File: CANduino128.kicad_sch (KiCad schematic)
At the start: 37 parts, among them J1 Conn_02x32_Row_Letter_First, J2 Conn_01x10, U1 AVR-H128-CAN, U2 74AHC373

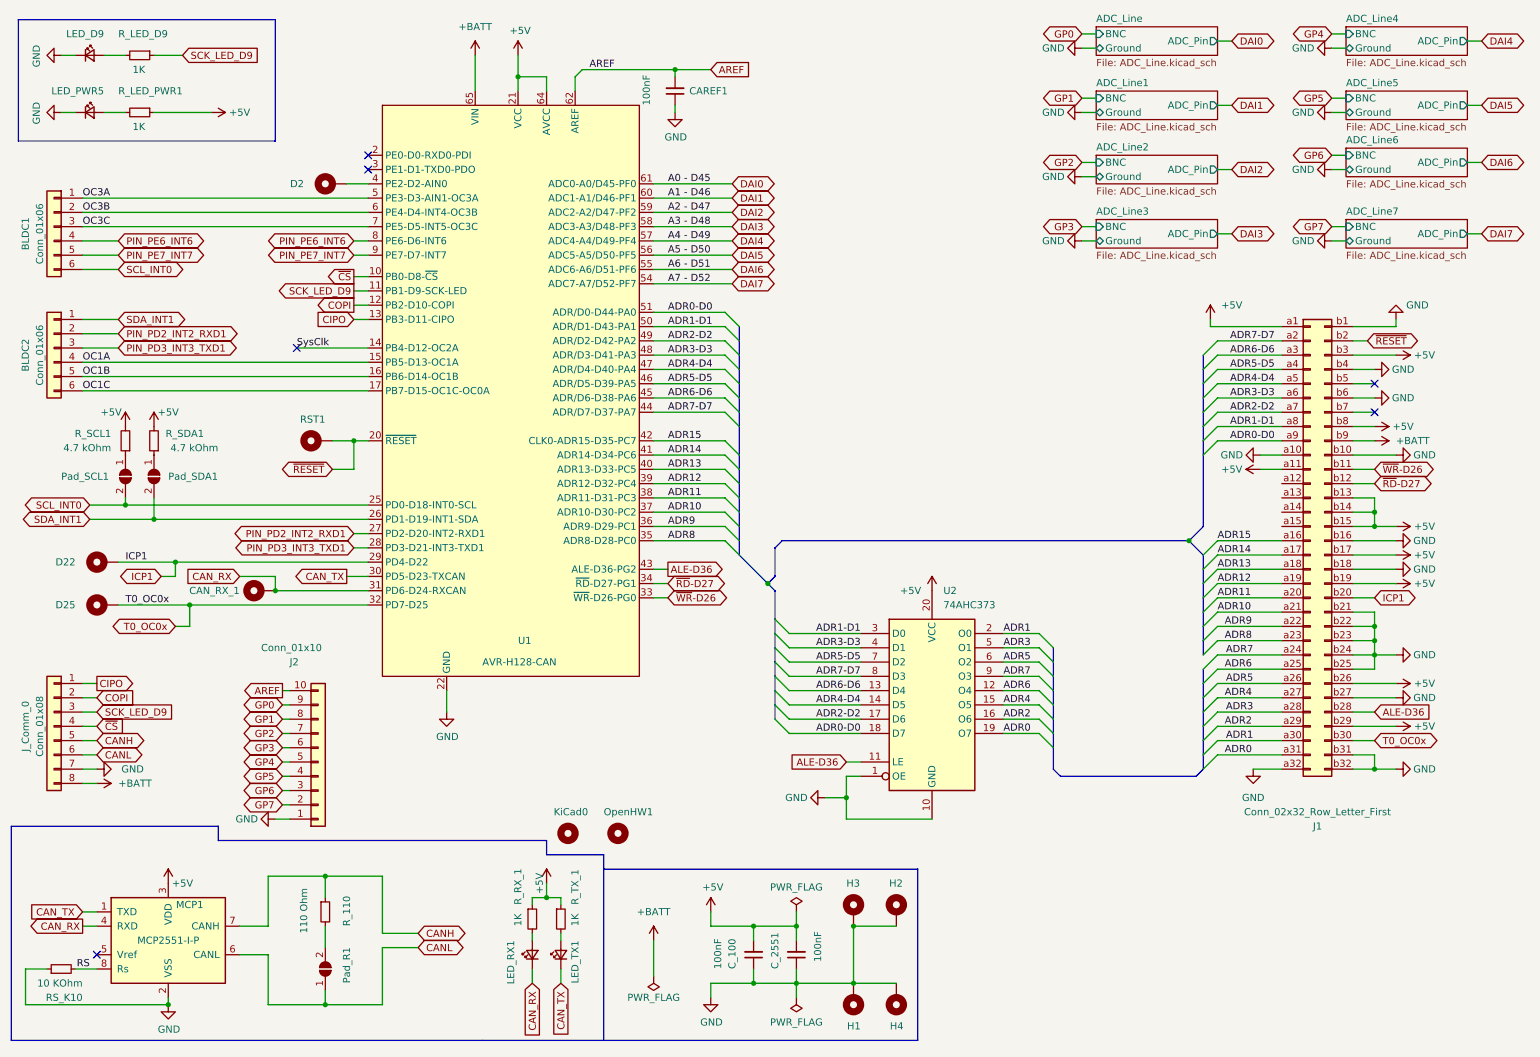
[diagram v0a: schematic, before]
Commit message: git-svn-id: file:///D%5C00%20-%20Dev%20&%20Calculs%5CRepoTortoiseSVN_PCB%5CCANduino128/branches/CANduino128%20-%20v3.x@78 67ddf66f-3787-a644-8df7-7746e21a92b3
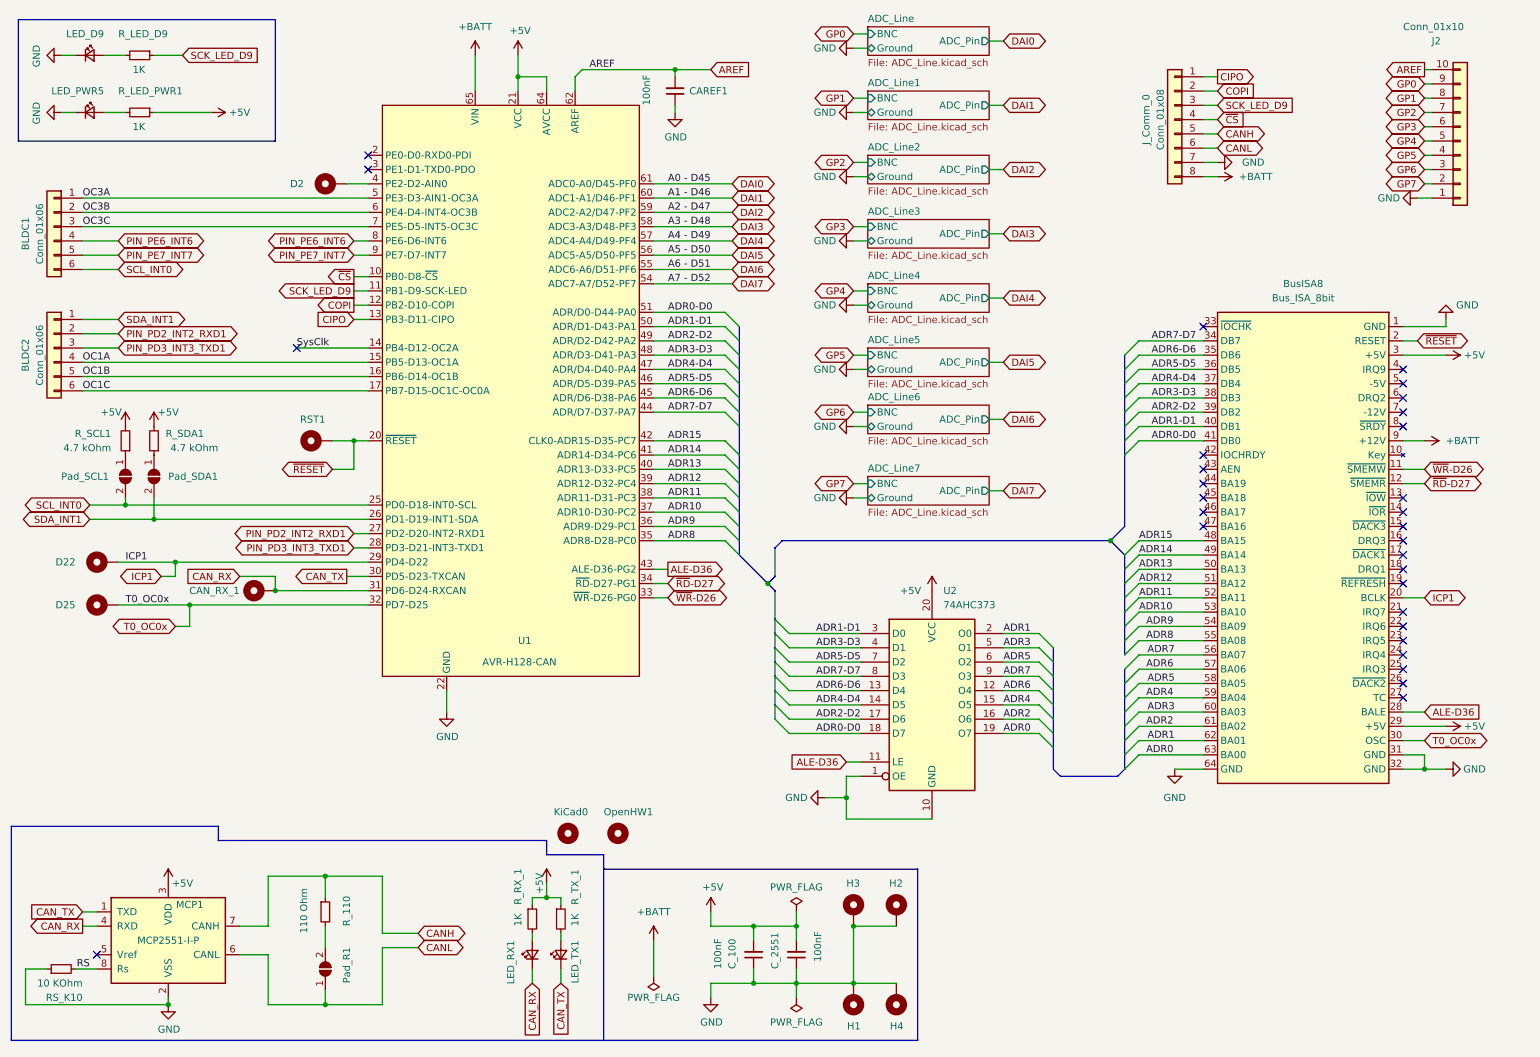
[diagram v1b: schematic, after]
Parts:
- removed J1: Conn_02x32_Row_Letter_First, AVR_H128-CAN:DIN41612_B_2x32_Female_Vertical_THT, symbol Connector_Generic:Conn_02x32_Row_Letter_First
- added BusISA8: Bus_ISA_8bit, Conn_ISA_8bits:PinSocket_2x32_P2.54mm_Vertical_TopBottom, symbol Conn_ISA_8bits:Bus_ISA_8bit
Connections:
- net +5V: now also BusISA8.29 (+5V), BusISA8.3 (+5V)
- net +BATT: now also BusISA8.9 (+12V)
- net ADR0: now also BusISA8.63 (BA00)
- net ADR0-D0: now also BusISA8.41 (DB0)
- net ADR1: now also BusISA8.62 (BA01)
- net ADR1-D1: now also BusISA8.40 (DB1)
- net ADR10: now also BusISA8.53 (BA10)
- net ADR11: now also BusISA8.52 (BA11)
- net ADR12: now also BusISA8.51 (BA12)
- net ADR13: now also BusISA8.50 (BA13)
- net ADR14: now also BusISA8.49 (BA14)
- net ADR15: now also BusISA8.48 (BA15)
- net ADR2: now also BusISA8.61 (BA02)
- net ADR2-D2: now also BusISA8.39 (DB2)
- net ADR3: now also BusISA8.60 (BA03)
- net ADR3-D3: now also BusISA8.38 (DB3)
- net ADR4: now also BusISA8.59 (BA04)
- net ADR4-D4: now also BusISA8.37 (DB4)
- net ADR5: now also BusISA8.58 (BA05)
- net ADR5-D5: now also BusISA8.36 (DB5)
- net ADR6: now also BusISA8.57 (BA06)
- net ADR6-D6: now also BusISA8.35 (DB6)
- net ADR7: now also BusISA8.56 (BA07)
- net ADR7-D7: now also BusISA8.34 (DB7)
- net ADR8: now also BusISA8.55 (BA08)
- net ADR9: now also BusISA8.54 (BA09)
- net ALE-D36: now also BusISA8.28 (BALE)
- net GND: now also BusISA8.1 (GND), BusISA8.31 (GND), BusISA8.32 (GND), BusISA8.64 (GND)
- net ICP1: now also BusISA8.20 (BCLK)
- net T0_OC0x: now also BusISA8.30 (OSC)
- net ~{RD}-D27: now also BusISA8.12 (~{SMEMR})
- net ~{RESET}: now also BusISA8.2 (RESET)
- net ~{WR}-D26: now also BusISA8.11 (~{SMEMW})
- no-connect marks 6 -> 30
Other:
- moved on the sheet: J2, J_Comm_0
